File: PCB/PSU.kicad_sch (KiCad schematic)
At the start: 76 parts, among them J2 Conn_01x02_Pin, J3 USB_C_Receptacle_USB2.0, J4 Conn_01x02_Pin, Q1 BC817, Q2 BC817, Q3 BC817, Q4 BC817, Q6 2N2219, SW2 SW_SPDT, SW3 SW_DPDT_x2, U1 BQ24075RGT, U2 BQ27441DRZR-G1A, U3 TPS63031DSK, U6 TPS63021DSJR, U7 LMS33460MG

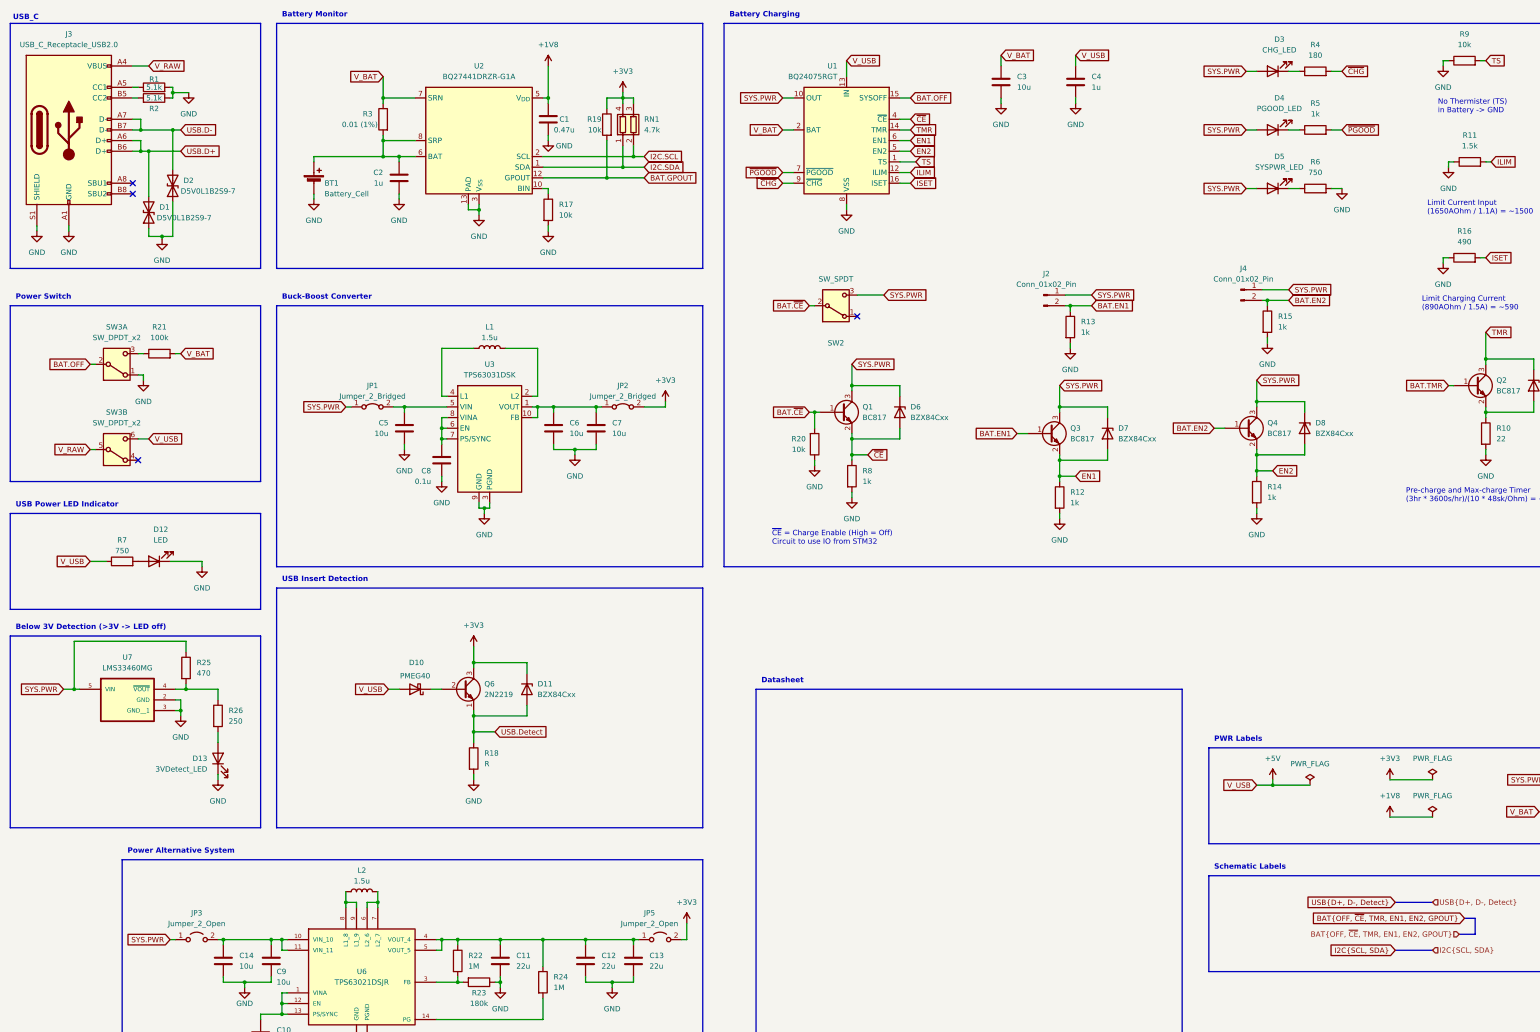
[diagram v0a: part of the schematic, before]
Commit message: PCB update - Minh
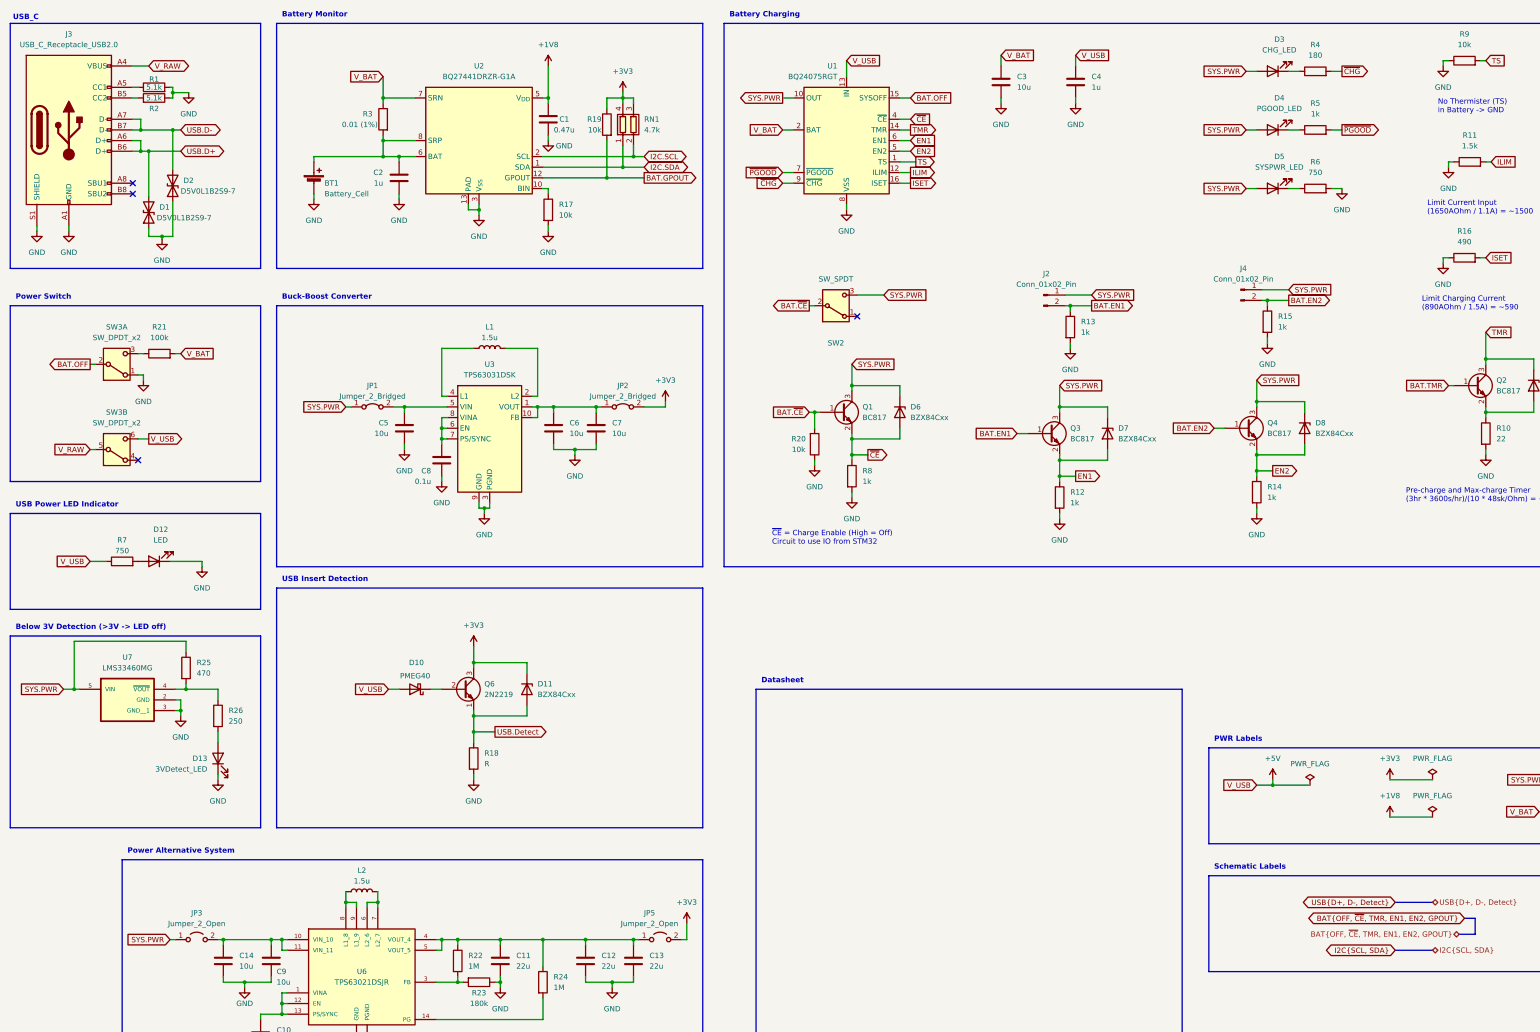
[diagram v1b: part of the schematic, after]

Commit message: Revert "PCB update - Minh"
This reverts commit 0608947e49f54a64abc006b190e3b029bac40ad1.
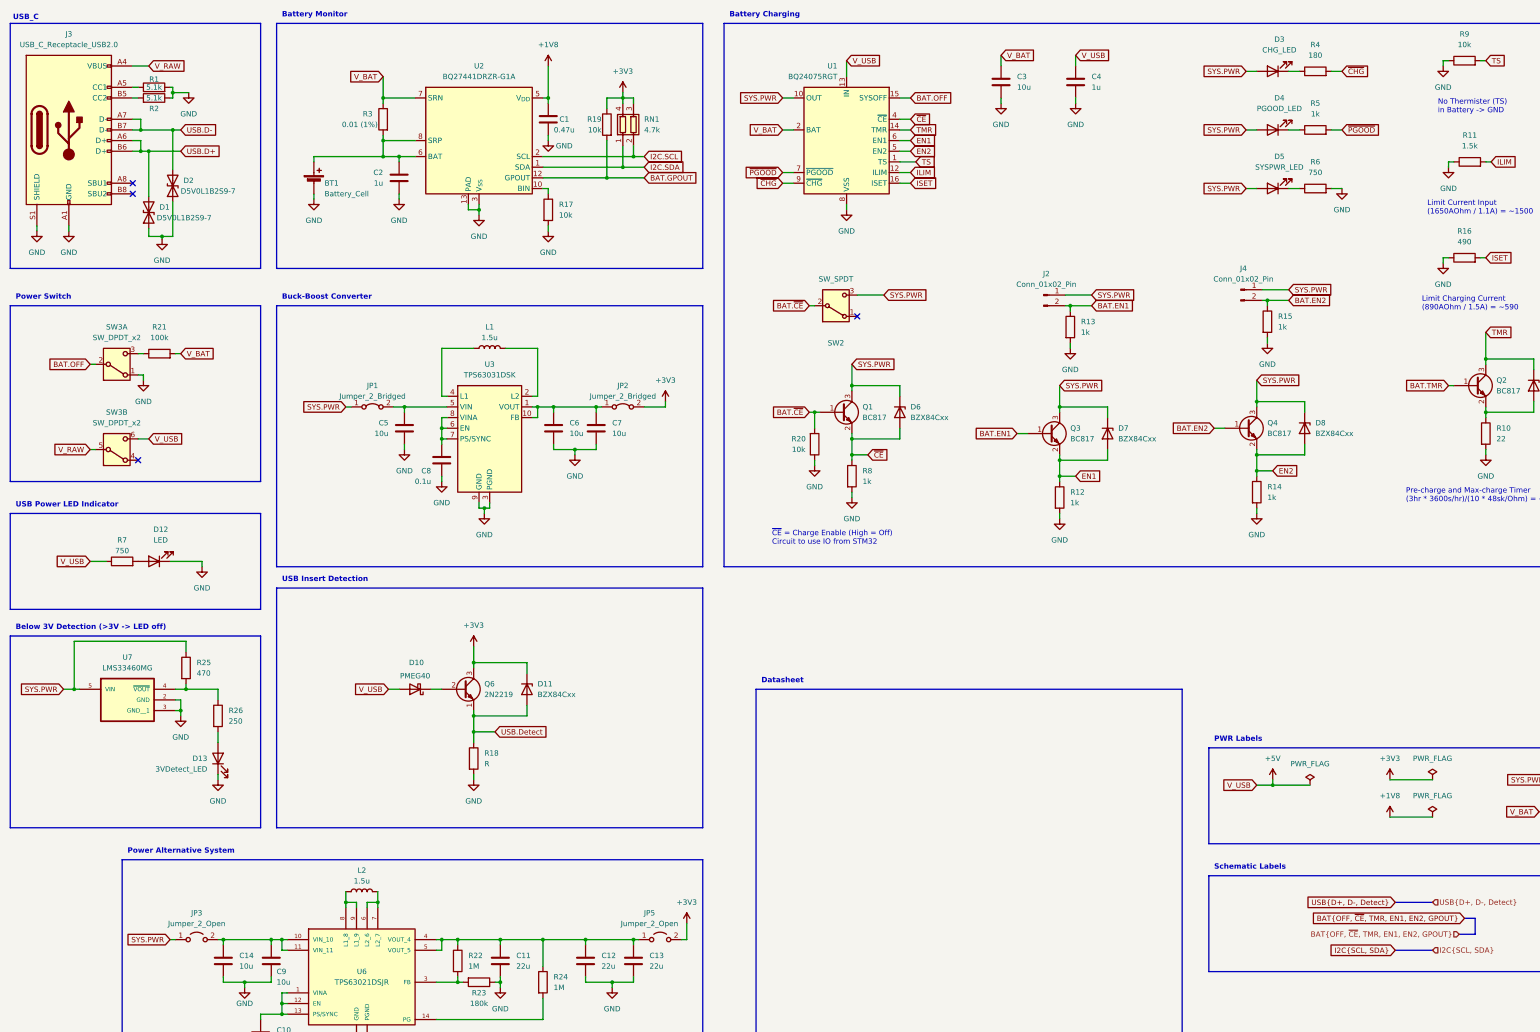
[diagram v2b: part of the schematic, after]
